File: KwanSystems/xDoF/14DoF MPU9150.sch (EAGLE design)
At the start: 18 parts, among them J401 M12PTH, U101 BMP180, U601 MPU9150, U901 ADXL377, U902 AD7991

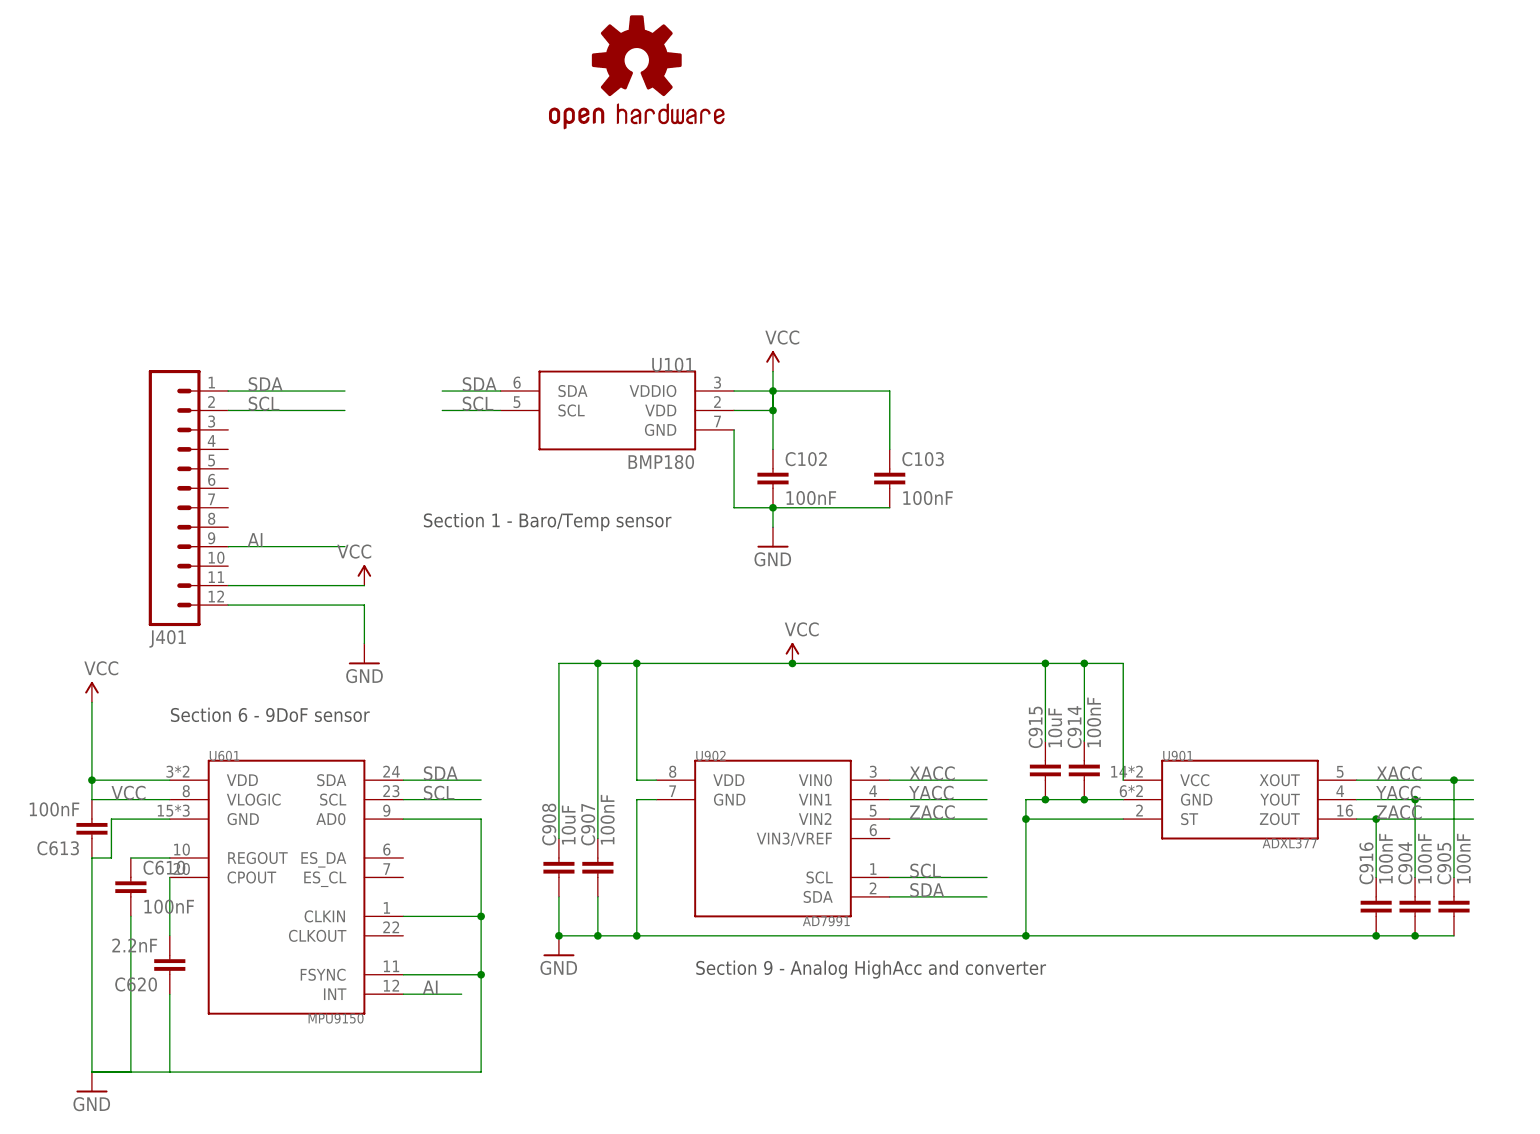
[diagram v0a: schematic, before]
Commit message: j
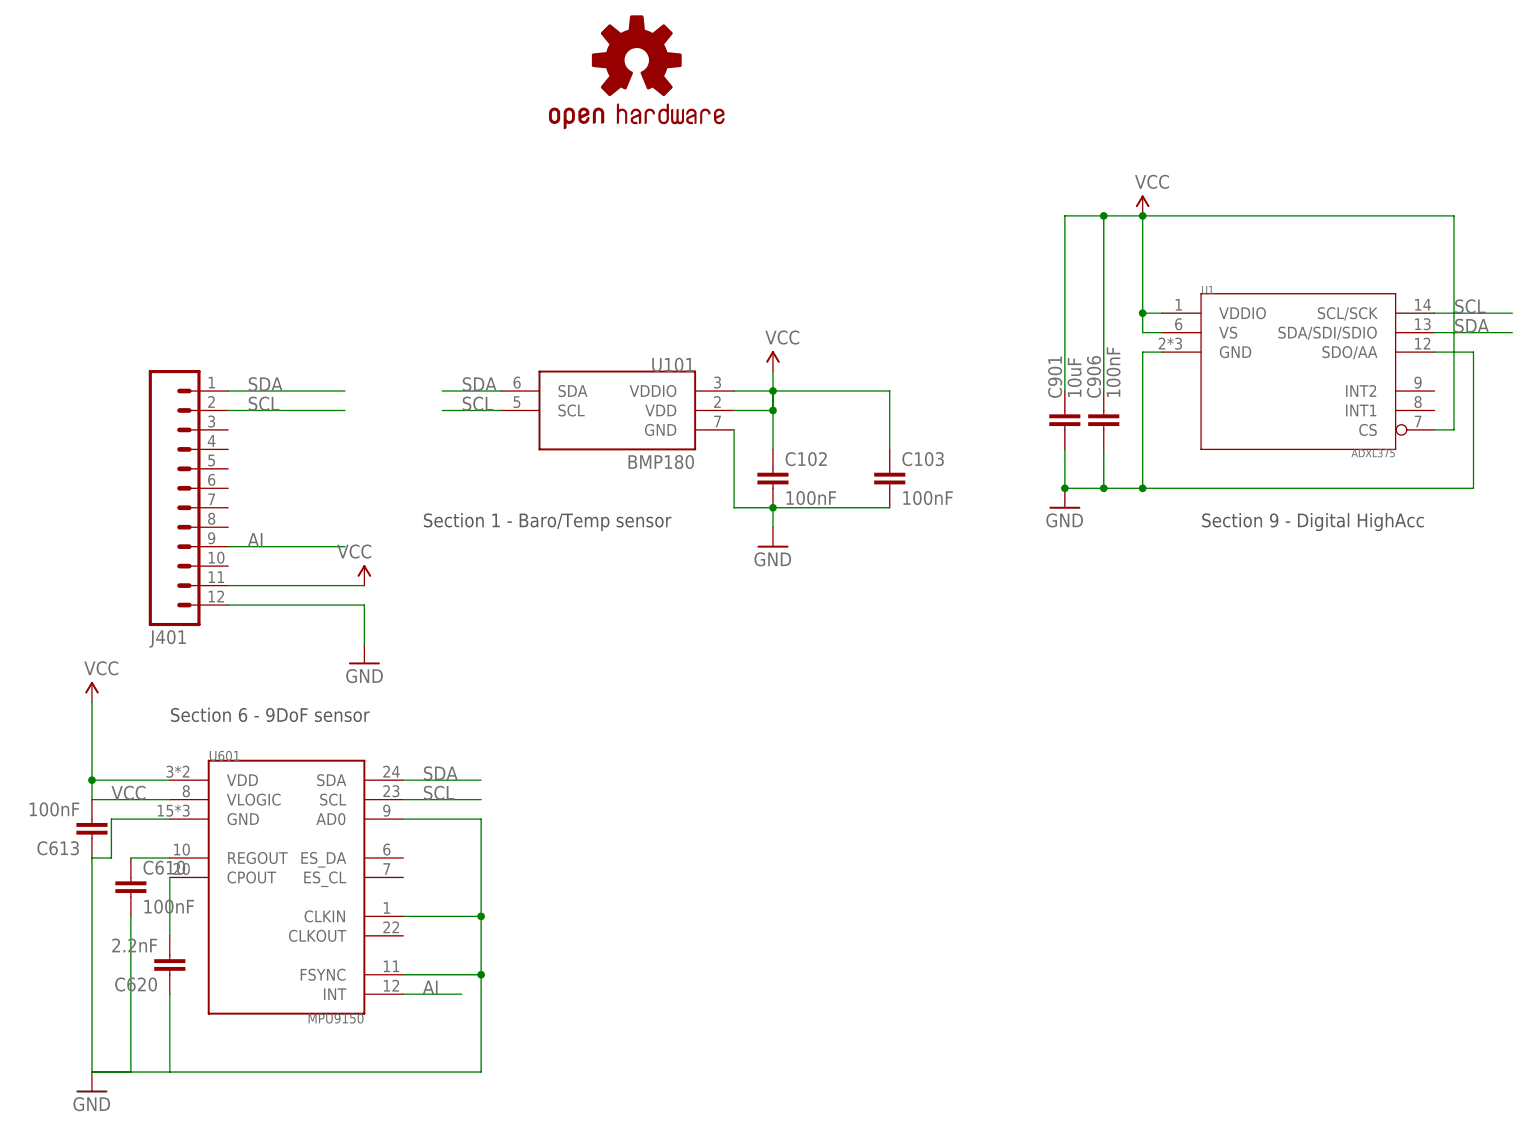
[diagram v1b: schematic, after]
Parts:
- removed C904, C905, C907, C914, C916: 100nF, SparkFun:CAP0603-CAP
- removed C908, C915: 10uF, SparkFun:CAP0603-CAP
- removed U901: ADXL377, KwanSystems:ADXL377
- removed U902: AD7991, KwanSystems:AD799X
- added C901: 10uF, SparkFun:CAP0603-CAP
- added C906: 100nF, SparkFun-Passives:CAP0402-CAP
- added U1: ADXL375, KwanSystems:ADXL375
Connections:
- removed net XACC: C905.1, U901.XOUT, U902.VIN0
- removed net YACC: C904.1, U901.YOUT, U902.VIN1
- removed net ZACC: C916.1, U901.ZOUT, U902.VIN2
- net GND: now also C901.2, C906.2, U1.GND, U1.SDO/AA; no longer C904.2, C905.2, C907.2, C908.2, C914.2, C915.2, C916.2, U901.GND, U901.ST, U902.GND
- net SCL: now also U1.SCL/SCK; no longer U902.SCL
- net SDA: now also U1.SDA/SDI/SDIO; no longer U902.SDA
- net VCC: now also C901.1, C906.1, U1.CS, U1.VDDIO, U1.VS; no longer C907.1, C908.1, C914.1, C915.1, U901.VCC, U902.VDD
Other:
- note added: "Section 9 - Digital HighAcc"
- note removed: "Section 9 - Analog HighAcc and converter"
